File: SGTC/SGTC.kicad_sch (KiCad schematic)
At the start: 1 part, among them J1 Conn_01x08_Pin

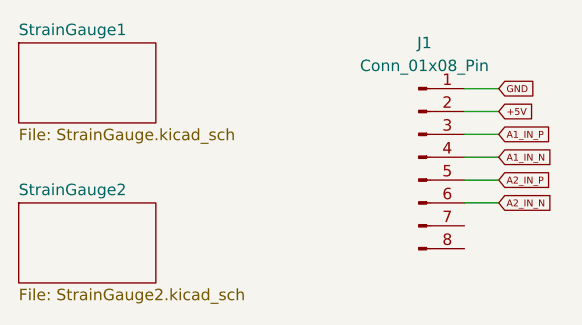
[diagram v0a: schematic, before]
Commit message: strain gauge fix
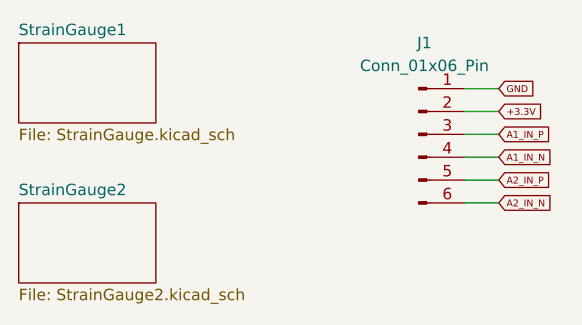
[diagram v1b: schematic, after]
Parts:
- removed J1: Conn_01x08_Pin, Connector_PinHeader_2.54mm:PinHeader_1x08_P2.54mm_Vertical, symbol Connector:Conn_01x08_Pin
- added J1: Conn_01x06_Pin, Connector_PinHeader_2.54mm:PinHeader_1x06_P2.54mm_Vertical, symbol Connector:Conn_01x06_Pin
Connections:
- net A1_IN_N: now also J1.4 (Pin_4)
- net A1_IN_P: now also J1.3 (Pin_3)
- net A2_IN_N: now also J1.6 (Pin_6)
- net A2_IN_P: now also J1.5 (Pin_5)
- net GND: now also J1.1 (Pin_1)
- new net +3.3V: J1.2 (Pin_2)
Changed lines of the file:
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@@
 		)
 	)
-	(global_label "+5V"
+	(global_label "+3.3V"
 		(shape input)
 		(at 179.07 72.39 0)
@@
 		)
 		(property "Intersheetrefs" "${INTERSHEET_REFS}"
-			(at 183.1836 72.39 0)
+			(at 184.2722 72.39 0)
 			(effects
 				(font
@@
 	)
 	(symbol
-		(lib_id "Connector:Conn_01x08_Pin")
-		(at 170.18 77.47 0)
+		(lib_id "Connector:Conn_01x06_Pin")
+		(at 170.18 74.93 0)
 		(unit 1)
 		(exclude_from_sim no)
@@
 			)
 		)
-		(property "Value" "Conn_01x08_Pin"
+		(property "Value" "Conn_01x06_Pin"
 			(at 170.815 67.31 0)
 			(effects
@@
 			)
 		)
-		(property "Footprint" "Connector_PinHeader_2.54mm:PinHeader_1x08_P2.54mm_Vertical"
-			(at 170.18 77.47 0)
+		(property "Footprint" "Connector_PinHeader_2.54mm:PinHeader_1x06_P2.54mm_Vertical"
+			(at 170.18 74.93 0)
 			(effects
 				(font
@@
 		)
 		(property "Datasheet" "~"
-			(at 170.18 77.47 0)
+			(at 170.18 74.93 0)
 			(effects
 				(font
@@
 			)
 		)
-		(property "Description" "Generic connector, single row, 01x08, script generated"
-			(at 170.18 77.47 0)
+		(property "Description" "Generic connector, single row, 01x06, script generated"
+			(at 170.18 74.93 0)
 			(effects
 				(font
@@
 			)
 		)
-		(pin "5"
+		(pin "4"
 		)
-		(pin "4"
+		(pin "1"
 		)
 		(pin "6"
 		)
-		(pin "8"
+		(pin "5"
+		)
+		(pin "2"
 		)
 		(pin "3"
 		)
-		(pin "7"
-		)
-		(pin "1"
-		)
-		(pin "2"
-		)
 		(instances
